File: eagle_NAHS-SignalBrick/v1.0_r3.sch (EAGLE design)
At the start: 45 parts, among them IC1 ESP12S, IC2 ATTINY212-SSNR, IC3 TP4056, IC4 DW01A, J1 10118194-0001LF, J2 BRICK-INTERF-V3_B-SIDE, Q1 8205A

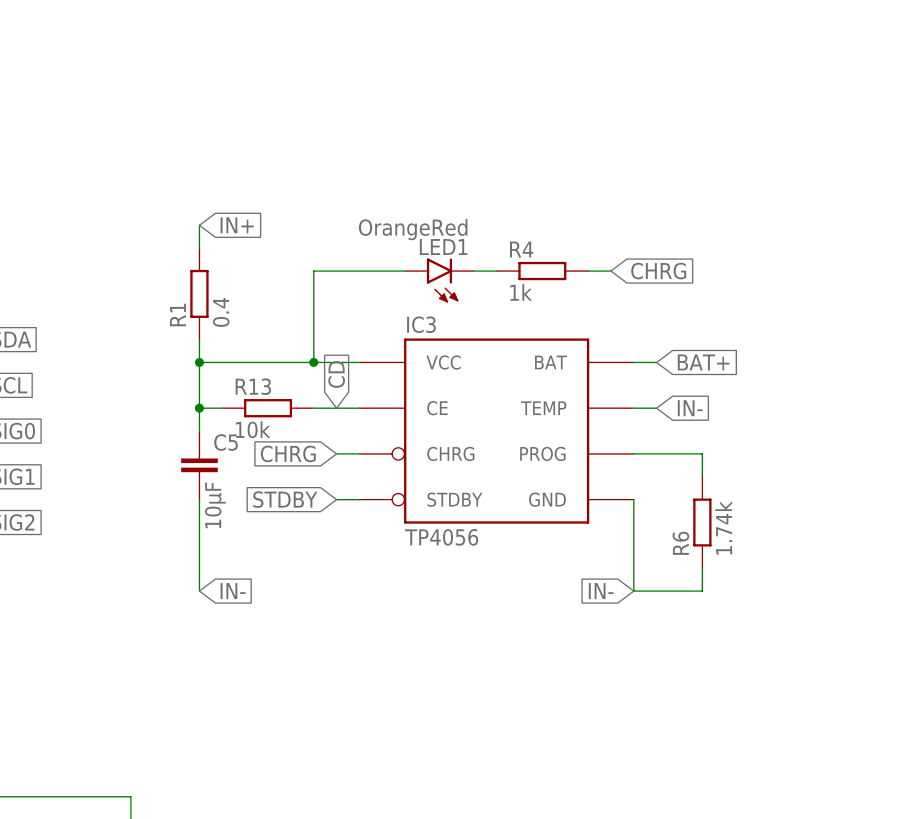
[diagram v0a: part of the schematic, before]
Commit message: Board v1.0 R3 WIP
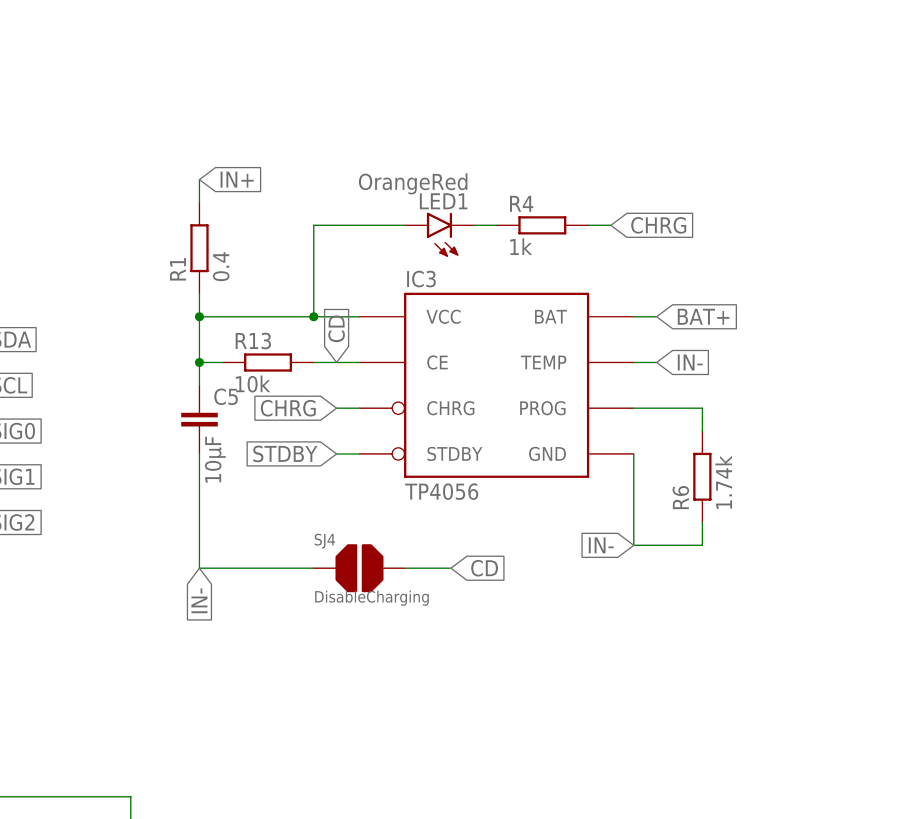
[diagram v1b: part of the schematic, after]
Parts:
- added SJ4: DisableCharging, no_pinhd:SOLDERJUMPER
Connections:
- net CD: now also SJ4.2
- net IN-: now also SJ4.1
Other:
- moved on the sheet: C5, IC3, LED1, R1, R13, R4, R6
